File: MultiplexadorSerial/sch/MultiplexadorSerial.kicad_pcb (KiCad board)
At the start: 2 copper layers, 69.2 x 53.9 mm, 68 parts, among them J1 SL, J2 SL1, J3 SL2, J4 SL3, J5 SL4, Q1 Q_NPN_CBE, Q2 Q_NPN_CBE, Q3 Q_NPN_CBE, Q4 Q_NPN_CBE, U1 SP3481CP, U2 4052, U3 SP3481CP, U4 SP3481CP, U5 SP3481CP

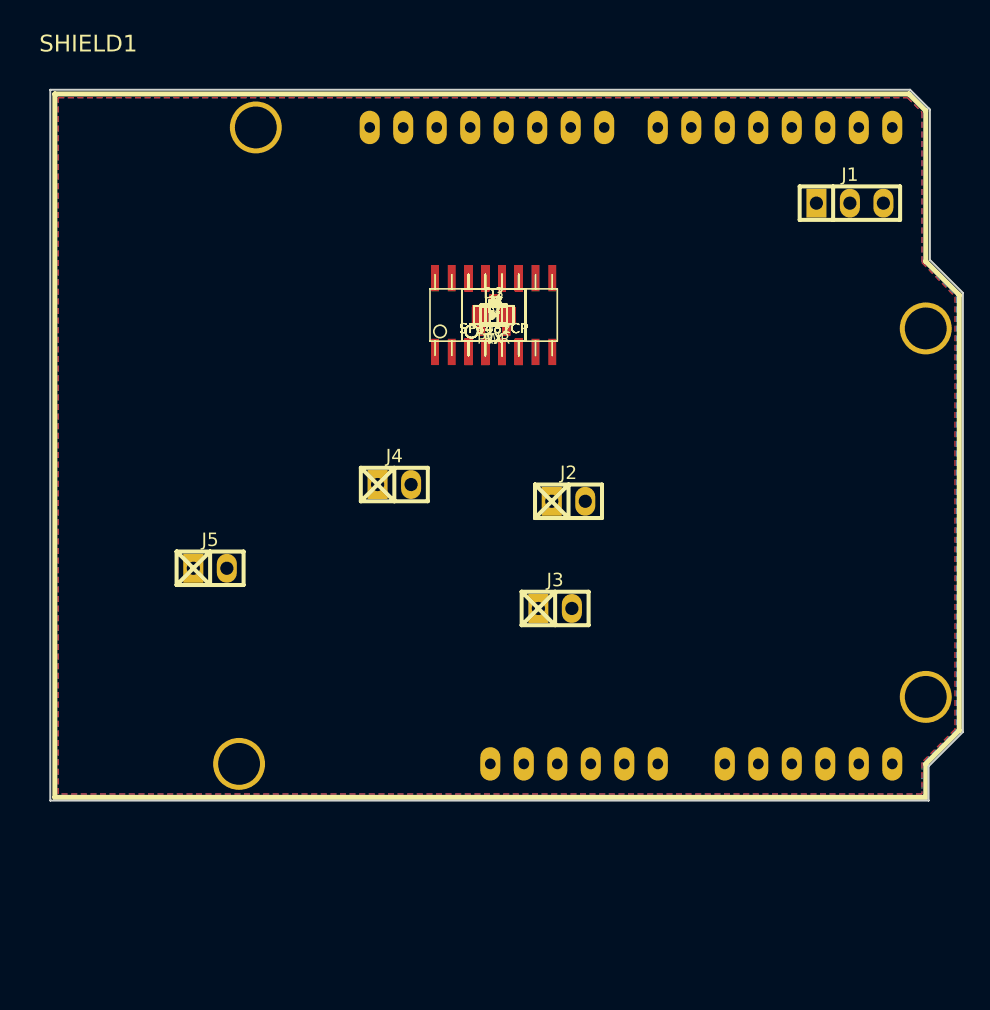
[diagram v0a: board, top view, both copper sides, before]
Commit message: Signed-off-by: cuki2 <mauricio@krebs.com.br>
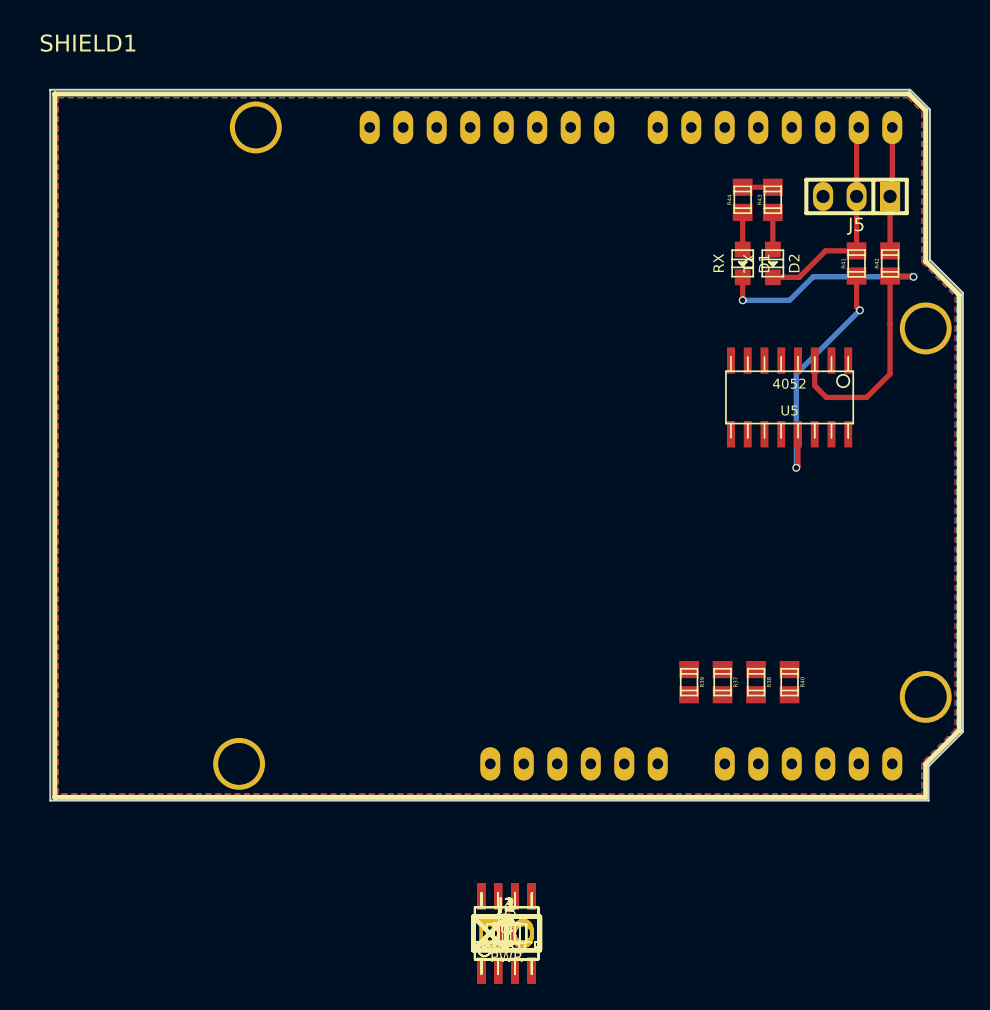
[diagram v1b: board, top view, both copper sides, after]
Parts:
- D1: value TX -> RX
- D2: value PWR -> TX
- D3: value RX -> PWR
- J1: value SL -> SL1; footprint w_pin_strip:pin_socket_3 -> w_pin_strip:pin_socket_2
- J2: value SL1 -> SL3
- J3: value SL2 -> SL4
- J4: value SL3 -> SL2
- J5: value SL4 -> SL; footprint w_pin_strip:pin_socket_2 -> w_pin_strip:pin_socket_3
- R1, R2: value 1k2 -> 10k
- R10: value 560R -> 360R
- R11, R26, R27: value 560R -> 10k
- R12: value 330R -> 10k
- R13: value 330R -> 120R
- R14, R33: value 10k -> 560R
- R15: value 10k -> 120R
- R16, R17: value 330R -> 560R
- R20, R24, R29, R3, R4: value 10k -> 360R
- R22, R23, R40, R6, R7: value 360R -> 10k
- R25, R9: value 120R -> 360R
- R31: value 360R -> 120R
- R32: value 360R -> 560R
- R37, R38, R42: value 10k -> 330R
- R41: value 360R -> 330R
- R43: value 120R -> 1k2
- R45: value 560R -> 1k2
- U2: value 4052 -> SP3481CP; footprint w_smd_dil:so-16 -> w_smd_dil:so-8
- U5: value SP3481CP -> 4052; footprint w_smd_dil:so-8 -> w_smd_dil:so-16
- moved J1 61.2 mm to (182.8, 115.3)
- moved J5 56.6 mm to (209.3, 59.4), turned to 180 degrees
- moved C1 46.9 mm to (182.8, 115.3)
- moved C2 46.9 mm to (182.8, 115.3)
- moved C3 46.9 mm to (182.8, 115.3)
- moved C4 46.9 mm to (182.8, 115.3)
- moved C5 46.9 mm to (182.8, 115.3)
- moved D3 46.9 mm to (182.8, 115.3)
- moved Q1 46.9 mm to (182.8, 115.3)
- moved Q2 46.9 mm to (182.8, 115.3)
- moved Q3 46.9 mm to (182.8, 115.3)
- moved Q4 46.9 mm to (182.8, 115.3)
- moved R1 46.9 mm to (182.8, 115.3)
- moved R10 46.9 mm to (182.8, 115.3)
- moved R11 46.9 mm to (182.8, 115.3)
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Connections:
- D1 pad 2: /TX -> Net-(D1-Pad2)
- D2 pad 1: +5V -> Net-(D2-Pad1)
- D2 pad 2: Net-(D2-Pad2) -> /TX
- D3 pad 1: Net-(D3-Pad1) -> +5V
- J1 pad 1: /TX -> Net-(J1-Pad1)
- J1 pad 2: /RX -> Net-(J1-Pad2)
- J5 pad 1: Net-(J5-Pad1) -> /RX
- J5 pad 2: Net-(J5-Pad2) -> /TX
- R1 pad 1: +5V -> Net-(Q1-Pad2)
- R1 pad 2: Net-(D1-Pad1) -> /RX1
- R10 pad 1: Net-(J2-Pad2) -> /TX3
- R10 pad 2: GND -> Net-(R10-Pad2)
- R11 pad 2: Net-(J2-Pad1) -> Net-(R11-Pad2)
- R12 pad 1: /ADR0 -> +5V
- R13 pad 1: /ADR1 -> Net-(J1-Pad1)
- R13 pad 2: Net-(R13-Pad2) -> Net-(J1-Pad2)
- R14 pad 1: GND -> Net-(J1-Pad2)
- R14 pad 2: Net-(R12-Pad2) -> GND
- R15 pad 1: GND -> Net-(J2-Pad1)
- R15 pad 2: Net-(R13-Pad2) -> Net-(J2-Pad2)
- R16 pad 1: /TX -> Net-(J2-Pad2)
- R16 pad 2: Net-(R16-Pad2) -> GND
- R17 pad 1: /RX -> +5V
- R17 pad 2: Net-(D3-Pad2) -> Net-(J1-Pad1)
- R18 pad 2: Net-(D3-Pad1) -> Net-(J2-Pad1)
- R19 pad 1: Net-(Q2-Pad2) -> Net-(Q3-Pad2)
- R19 pad 2: /RX2 -> /RX4
- R2 pad 1: GND -> Net-(Q2-Pad2)
- R2 pad 2: Net-(D2-Pad2) -> /RX3
- R20 pad 1: +5V -> /RX4
- R20 pad 2: Net-(Q2-Pad3) -> Net-(R20-Pad2)
- R21 pad 1: /TX2 -> /TX4
- R22 pad 1: /RX2 -> Net-(Q4-Pad2)
- R22 pad 2: Net-(R22-Pad2) -> /RX2
- R23 pad 1: /TX2 -> +5V
- R23 pad 2: Net-(R23-Pad2) -> Net-(Q3-Pad3)
- R24 pad 1: +5V -> /TX4
- R24 pad 2: Net-(R22-Pad2) -> Net-(R24-Pad2)
- R25 pad 1: Net-(J3-Pad1) -> /RX2
- R25 pad 2: Net-(J3-Pad2) -> Net-(R25-Pad2)
- R26 pad 1: Net-(J3-Pad2) -> +5V
- R26 pad 2: GND -> Net-(R20-Pad2)
- R27 pad 1: +5V -> /TX2
- R27 pad 2: Net-(J3-Pad1) -> +5V
- R28 pad 1: Net-(Q3-Pad2) -> +5V
- R28 pad 2: /RX3 -> Net-(Q4-Pad3)
- R29 pad 1: +5V -> /TX2
- R29 pad 2: Net-(Q3-Pad3) -> Net-(R29-Pad2)
- R3 pad 1: Net-(Q1-Pad2) -> /RX1
- R3 pad 2: /RX1 -> Net-(R11-Pad2)
- R30 pad 1: /TX3 -> +5V
- R30 pad 2: +5V -> Net-(R25-Pad2)
- R31 pad 1: /RX3 -> Net-(J3-Pad1)
- R31 pad 2: Net-(R31-Pad2) -> Net-(J3-Pad2)
- R32 pad 1: /TX3 -> Net-(J3-Pad2)
- R32 pad 2: Net-(R32-Pad2) -> GND
- R33 pad 2: Net-(R31-Pad2) -> Net-(J3-Pad1)
- R37 pad 1: Net-(Q4-Pad2) -> /ADR0
- R37 pad 2: /RX4 -> Net-(R37-Pad2)
- R38 pad 1: +5V -> /ADR1
- R38 pad 2: Net-(Q4-Pad3) -> Net-(R38-Pad2)
- R39 pad 1: /TX4 -> GND
- R39 pad 2: +5V -> Net-(R37-Pad2)
- R4 pad 1: +5V -> /RX3
- R4 pad 2: Net-(Q1-Pad3) -> Net-(R12-Pad2)
- R40 pad 1: /RX4 -> GND
- R40 pad 2: Net-(R40-Pad2) -> Net-(R38-Pad2)
- R41 pad 1: /TX4 -> /TX
- R42 pad 1: +5V -> /RX
- R42 pad 2: Net-(R40-Pad2) -> Net-(D1-Pad2)
- R43 pad 1: Net-(J5-Pad1) -> +5V
- R43 pad 2: Net-(J5-Pad2) -> Net-(D2-Pad1)
- R44 pad 1: Net-(J5-Pad2) -> +5V
- R44 pad 2: GND -> Net-(D1-Pad1)
- R45 pad 1: +5V -> GND
- R45 pad 2: Net-(J5-Pad1) -> Net-(D3-Pad2)
- R6 pad 1: /RX1 -> /TX3
- R6 pad 2: Net-(R6-Pad2) -> +5V
- R7 pad 1: /TX1 -> +5V
- R7 pad 2: Net-(R7-Pad2) -> Net-(Q1-Pad3)
- R8 pad 2: Net-(R6-Pad2) -> Net-(Q2-Pad3)
- R9 pad 1: Net-(J2-Pad1) -> /TX1
- R9 pad 2: Net-(J2-Pad2) -> Net-(R9-Pad2)
- U1 pad 1: Net-(R6-Pad2) -> Net-(R11-Pad2)
- U1 pad 4: Net-(R7-Pad2) -> Net-(R9-Pad2)
- U1 pad 6: Net-(J2-Pad1) -> Net-(J1-Pad1)
- U1 pad 7: Net-(J2-Pad2) -> Net-(J1-Pad2)
- U2 pad 1: /RX1 -> Net-(R12-Pad2)
- U2 pad 2: /RX3 -> Net-(Q2-Pad3)
- U2 pad 3: Net-(D3-Pad2) -> Net-(Q2-Pad3)
- U2 pad 4: /RX4 -> Net-(R10-Pad2)
- U2 pad 5: /RX2 -> GND
- U2 pad 6: GND -> Net-(J2-Pad1)
- U2 pad 7: GND -> Net-(J2-Pad2)
- U2 pad 8: GND -> +5V
- U3 pad 1: Net-(R22-Pad2) -> Net-(R20-Pad2)
- U3 pad 2: Net-(Q2-Pad3) -> Net-(Q3-Pad3)
- U3 pad 3: Net-(Q2-Pad3) -> Net-(Q3-Pad3)
- U3 pad 4: Net-(R23-Pad2) -> Net-(R24-Pad2)
- U4 pad 1: Net-(R31-Pad2) -> Net-(R25-Pad2)
- U4 pad 2: Net-(Q3-Pad3) -> Net-(Q4-Pad3)
- U4 pad 3: Net-(Q3-Pad3) -> Net-(Q4-Pad3)
- U4 pad 4: Net-(R32-Pad2) -> Net-(R29-Pad2)
- U5 pad 1: Net-(R40-Pad2) -> /RX1
- U5 pad 2: Net-(Q4-Pad3) -> /RX3
- U5 pad 3: Net-(Q4-Pad3) -> Net-(D1-Pad2)
- U5 pad 4: Net-(R41-Pad2) -> /RX4
- U5 pad 5: GND -> /RX2
- U5 pad 6: Net-(J5-Pad1) -> GND
- U5 pad 7: Net-(J5-Pad2) -> GND
- U5 pad 8: +5V -> GND
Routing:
- net Net-(D1-Pad2): track 0.00 -> 33.4 mm, vias 0 -> 2
- net Net-(R41-Pad2): track 0.00 -> 19.2 mm, vias 0 -> 2
- net /TX: track 0.00 -> 16.6 mm
- net /RX: track 0.00 -> 9.43 mm
- net Net-(D2-Pad1): track 0.00 -> 2.82 mm
- net Net-(D1-Pad1): track 0.00 -> 2.82 mm
- net +5V: track 0.00 -> 2.29 mm
